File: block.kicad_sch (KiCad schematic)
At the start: 97 parts, among them SW1 SW_PUSH, SW10 SW_PUSH, SW11 SW_PUSH, SW12 SW_PUSH, SW13 SW_PUSH, SW14 SW_PUSH, SW15 SW_PUSH, SW16 SW_PUSH, SW17 SW_PUSH, SW18 SW_PUSH, SW19 SW_PUSH, SW2 SW_PUSH, SW20 SW_PUSH, SW21 SW_PUSH, SW22 SW_PUSH, SW23 SW_PUSH, SW24 SW_PUSH, SW25 SW_PUSH, SW26 SW_PUSH, SW27 SW_PUSH, SW28 SW_PUSH, SW29 SW_PUSH, SW3 SW_PUSH, SW30 SW_PUSH, SW31 SW_PUSH, SW32 SW_PUSH, SW33 SW_PUSH, SW34 SW_PUSH, SW35 SW_PUSH, SW36 SW_PUSH, SW37 SW_PUSH, SW38 SW_PUSH, SW39 SW_PUSH, SW4 SW_PUSH, SW40 SW_PUSH, SW41 SW_PUSH, SW42 SW_PUSH, SW43 SW_PUSH, SW44 SW_PUSH, SW45 SW_PUSH, SW46 SW_PUSH, SW47 SW_PUSH, SW48 SW_PUSH, SW5 SW_PUSH, SW6 SW_PUSH, SW7 SW_PUSH, SW8 SW_PUSH, SW9 SW_PUSH, U1 ProMicro

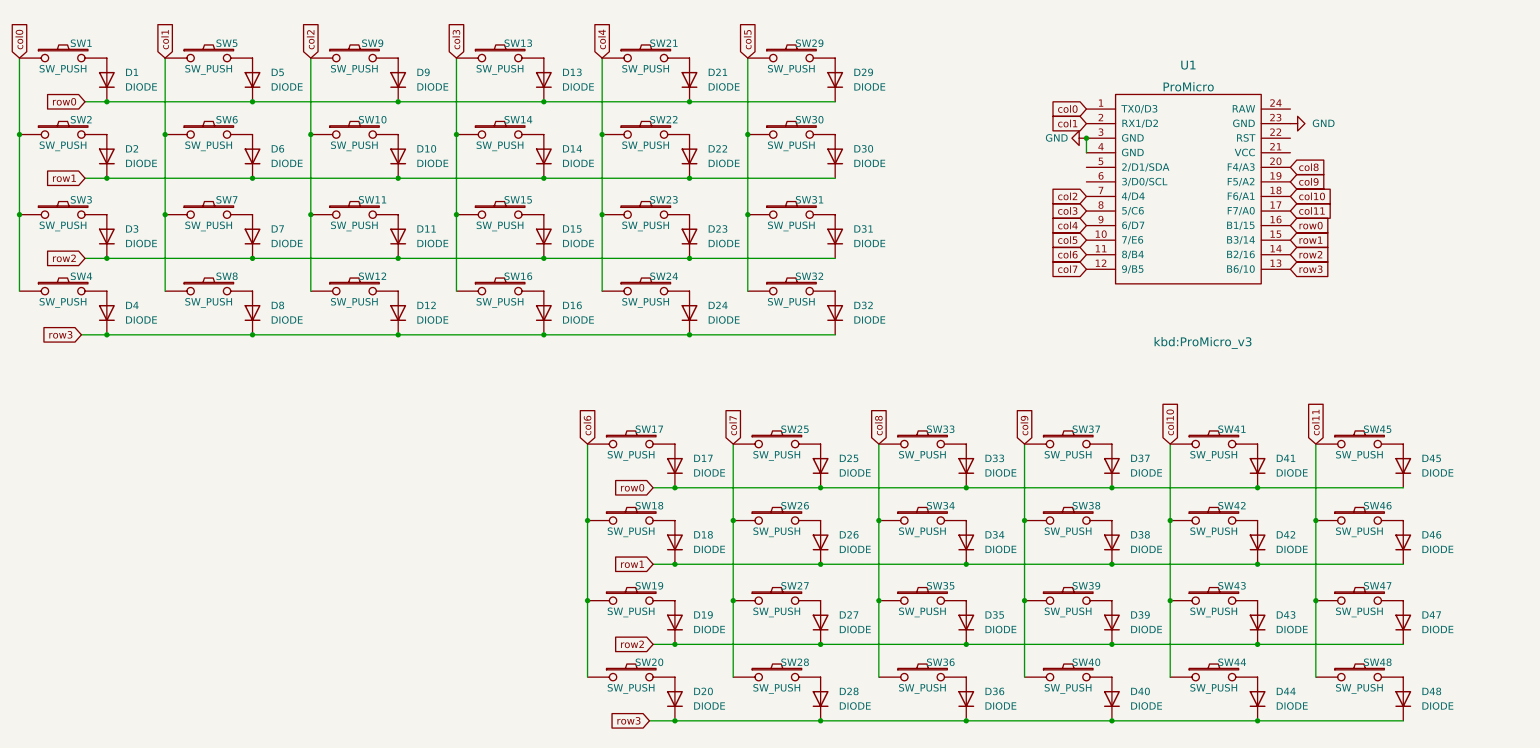
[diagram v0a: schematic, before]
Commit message: block board
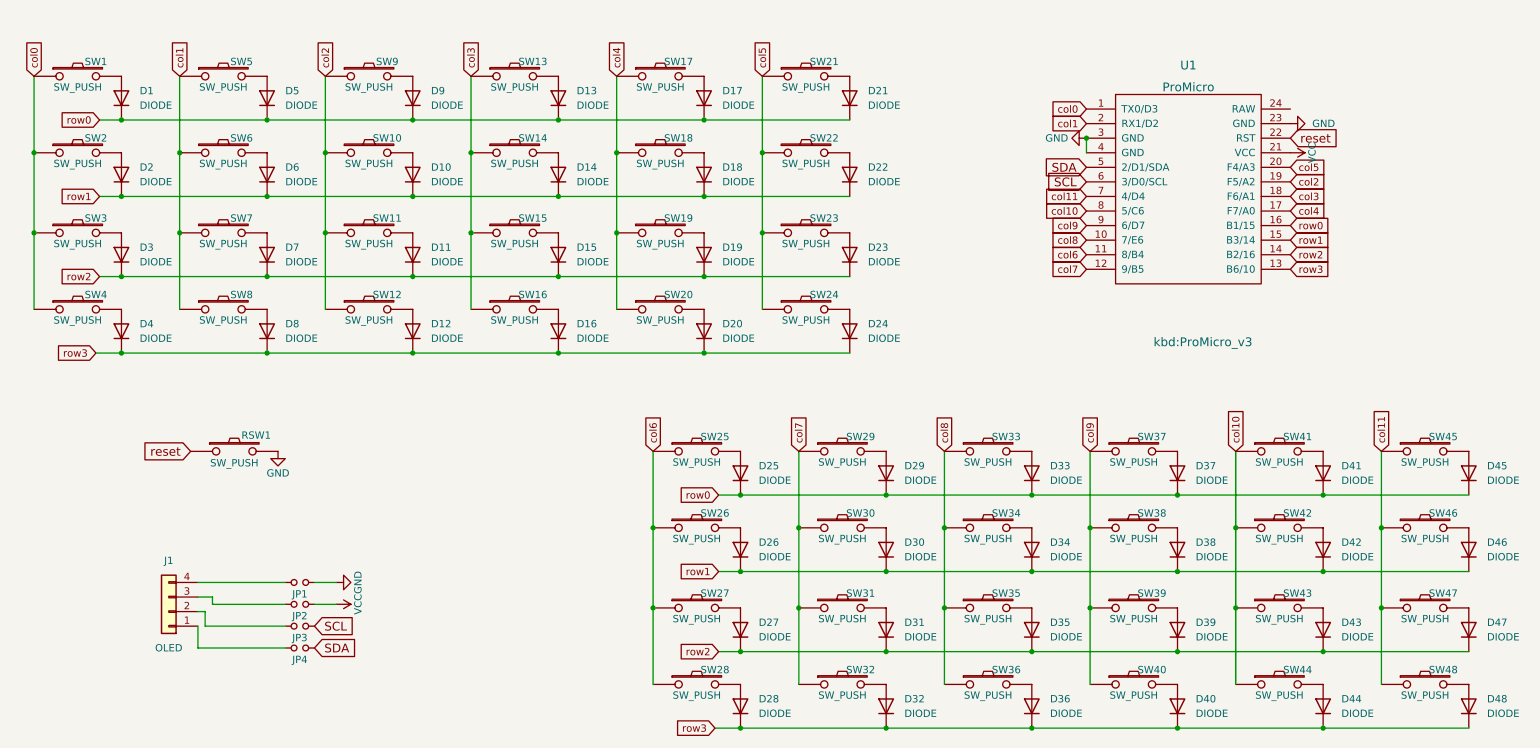
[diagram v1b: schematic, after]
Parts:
- added J1: OLED, kbd:OLED, symbol Connector_Generic:Conn_01x04
- added JP1, JP2, JP3, JP4: (no value), kbd:Jumper, symbol corne-chocolate-rescue:Jumper_NO_Small-Device
- added RSW1: SW_PUSH, kbd:ResetSW_1side, symbol corne-chocolate-rescue:SW_PUSH-kbd
- renumbered D21 to D17, D22 to D18, D23 to D19, D24 to D20, D29 to D21, D30 to D22, D31 to D23, D32 to D24, D17 to D25, D18 to D26, D19 to D27, D20 to D28, D25 to D29, D26 to D30, D27 to D31, D28 to D32, SW21 to SW17, SW22 to SW18, SW23 to SW19, SW24 to SW20, SW29 to SW21, SW30 to SW22, SW31 to SW23, SW32 to SW24, SW17 to SW25, SW18 to SW26, SW19 to SW27, SW20 to SW28, SW25 to SW29, SW26 to SW30, SW27 to SW31, SW28 to SW32
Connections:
- net GND: now also JP1.1, RSW1.2
- net col10: now also U1.8 (5/C6); no longer U1.18 (F6/A1)
- net col11: now also U1.7 (4/D4); no longer U1.17 (F7/A0)
- net col2: now also U1.19 (F5/A2); no longer U1.7 (4/D4)
- net col3: now also U1.18 (F6/A1); no longer U1.8 (5/C6)
- net col4: now also U1.17 (F7/A0); no longer U1.9 (6/D7)
- net col5: now also U1.20 (F4/A3); no longer U1.10 (7/E6)
- net col8: now also U1.10 (7/E6); no longer U1.20 (F4/A3)
- net col9: now also U1.9 (6/D7); no longer U1.19 (F5/A2)
- net VCC: now reaches U1.21 (VCC)
- net VCC: now also JP2.1
- net reset: now reaches U1.22 (RST)
- net reset: now also RSW1.1
- net SDA: now reaches U1.5 (2/D1/SDA)
- net SDA: now also JP4.1
- net SCL: now reaches U1.6 (3/D0/SCL)
- net SCL: now also JP3.1
- new net: J1.2 (Pin_2), JP3.2
- new net: J1.3 (Pin_3), JP2.2
- new net: J1.4 (Pin_4), JP1.2
- new net: J1.1 (Pin_1), JP4.2
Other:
- moved on the sheet: D1, D10, D11, D12, D13, D14, D15, D16, D17, D18, D19, D2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

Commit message: mounting holes
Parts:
- D1, D10, D11, D12, D13, D14, D15, D16, D17, D18, D19, D2, D20, D21, D22, D23, D24, D25, D26, D27, D28, D29, D3, D30, D31, D32, D33, D34, D35, D36, D37, D38, D39, D4, D40, D41, D42, D43, D44, D45, D46, D47, D48, D5, D6, D7, D8, D9: footprint kbd:D3_TH_SMD_v2 -> kbd:D3_SMD_v2
